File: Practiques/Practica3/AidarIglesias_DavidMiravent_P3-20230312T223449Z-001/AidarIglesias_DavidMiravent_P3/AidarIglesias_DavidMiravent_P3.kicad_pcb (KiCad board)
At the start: 4 copper layers, 53.3 x 31.3 mm, 32 parts, among them IC1 PIC18F258-I_SO, J1 ANALOG INPUT, J2 Screw_Terminal_01x02, J3 PROGRAMMING CON, J4 JP2, J5 JP1, J6 USART CON, SW1 SW_Push, U1 LT1492, U2 LM1117-ADJ, Y1 ABLS2-16.000MHZ-D4Y-T

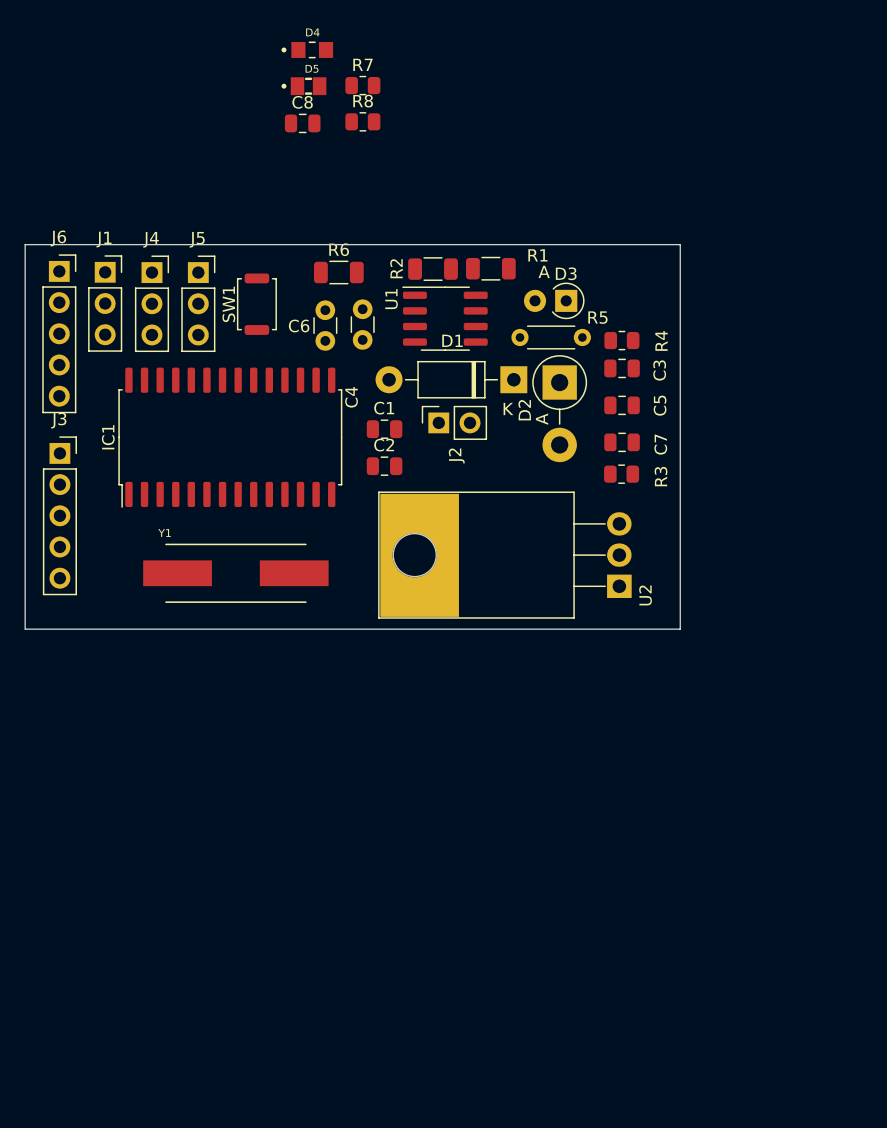
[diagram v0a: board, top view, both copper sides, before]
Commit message: Mod_14_03_23_00_44
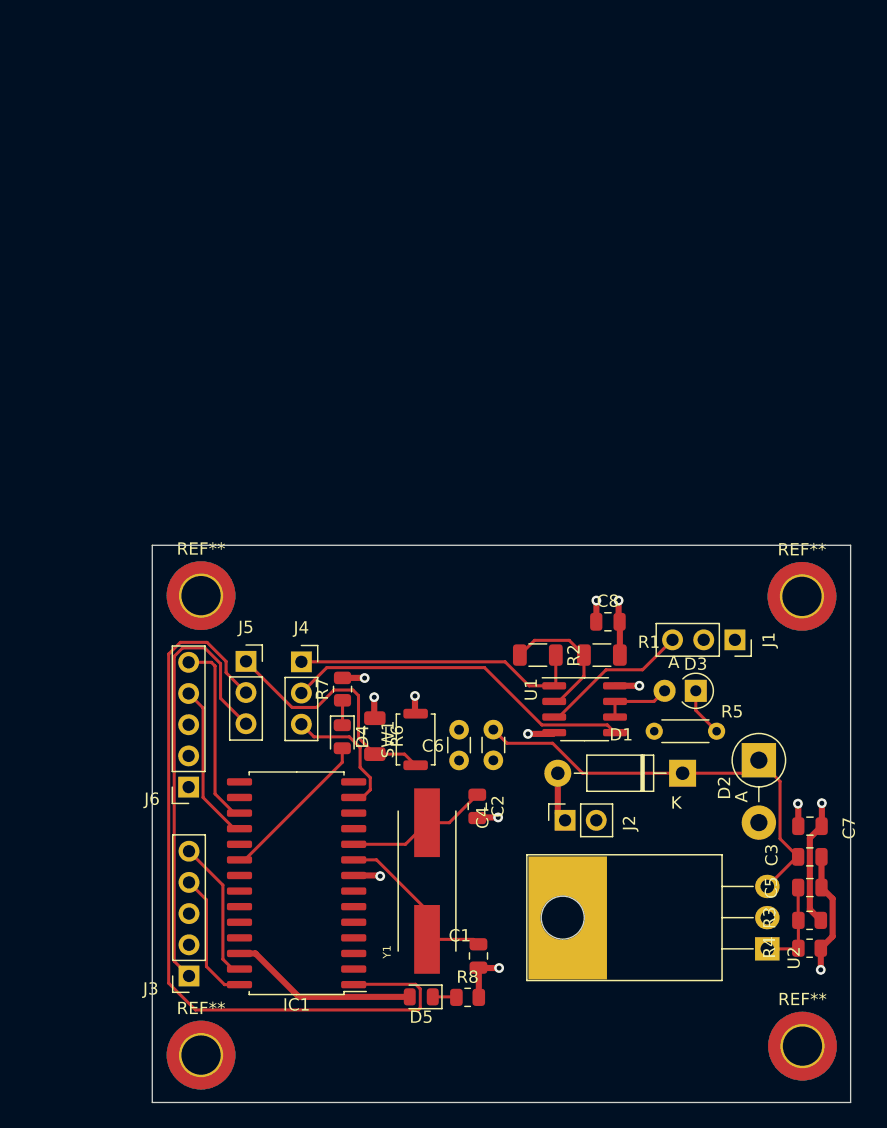
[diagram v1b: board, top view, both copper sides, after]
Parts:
- added REF**: MountingHole_3.2mm_M3_DIN965_Pad_TopBottom, MountingHole:MountingHole_3.2mm_M3_DIN965_Pad_TopBottom, F.Cu at (146.9, 79.4)
- added REF**: MountingHole_3.2mm_M3_DIN965_Pad_TopBottom, MountingHole:MountingHole_3.2mm_M3_DIN965_Pad_TopBottom, F.Cu at (98.0, 116.7)
- added REF**: MountingHole_3.2mm_M3_DIN965_Pad_TopBottom, MountingHole:MountingHole_3.2mm_M3_DIN965_Pad_TopBottom, F.Cu at (98.0, 79.3)
- added REF**: MountingHole_3.2mm_M3_DIN965_Pad_TopBottom, MountingHole:MountingHole_3.2mm_M3_DIN965_Pad_TopBottom, F.Cu at (146.9, 116.0)
- D4: footprint LED_SMD:LED_7012X1 -> LED_SMD:LED_0805_2012Metric
- D5: footprint LED_SMD:LEDC2012X70N -> LED_SMD:LED_0805_2012Metric
- moved D5 74.7 mm to (115.9, 112.0), turned to 180 degrees
- moved R8 71.8 mm to (119.7, 112.0)
- moved J1 59.4 mm to (141.4, 82.9), turned to -90 degrees
- moved D4 56.0 mm to (109.5, 90.8), turned to -90 degrees
- moved R4 51.8 mm to (147.5, 108.0), turned to 0 degrees
- moved R7 49.2 mm to (109.5, 86.9), turned to 90 degrees
- moved C8 47.6 mm to (131.1, 81.4)
- moved J3 43.8 mm to (97.0, 110.3), turned to 180 degrees
- moved C1 43.6 mm to (120.6, 108.7), turned to -90 degrees
- moved J6 43.3 mm to (97.0, 94.9), turned to 180 degrees
- moved C3 42.6 mm to (147.5, 100.6), turned to 0 degrees
- moved C5 42.1 mm to (147.5, 103.1), turned to 0 degrees
- moved R3 39.4 mm to (147.5, 105.8), turned to 180 degrees
- moved R6 37.9 mm to (112.1, 90.8), turned to -90 degrees
- moved SW1 37.7 mm to (115.4, 91.0)
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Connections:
- R7 pad 1: /Vlr -> /Vledr
- R8 pad 1: /Vlb -> /Vledb
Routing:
- net MCLR: track 0.00 -> 64.3 mm
- net PROG_MCLR: track 0.00 -> 36.9 mm
- net /V_{in}: track 0.00 -> 36.2 mm
- net Vdrive: track 0.00 -> 28.6 mm
- net GND: track 0.00 -> 28.0 mm, vias 0 -> 8
- net /VAMP: track 0.00 -> 24.9 mm
- net /Vsw: track 0.00 -> 20.5 mm
- net +VCC: track 0.00 -> 17.6 mm, vias 0 -> 5
- net PGM: track 0.00 -> 15.3 mm
- net TX: track 0.00 -> 15.3 mm
- net XTAL1: track 0.00 -> 14.4 mm
- net RX: track 0.00 -> 13.0 mm
- net /Vdd: track 0.00 -> 12.8 mm
- net Vin: track 0.00 -> 12.2 mm
- net XTAL2: track 0.00 -> 11.7 mm
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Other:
- board size 53.3 x 31.3 mm -> 56.9 x 45.4 mm
